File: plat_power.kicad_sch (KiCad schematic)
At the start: 56 parts, among them Con2 DG125-5.0-02P-14-00A(H), U1 LD39050PU33R, U2 TPS5450, U3 TPS5450, U4 TPS5450, con3 KF202

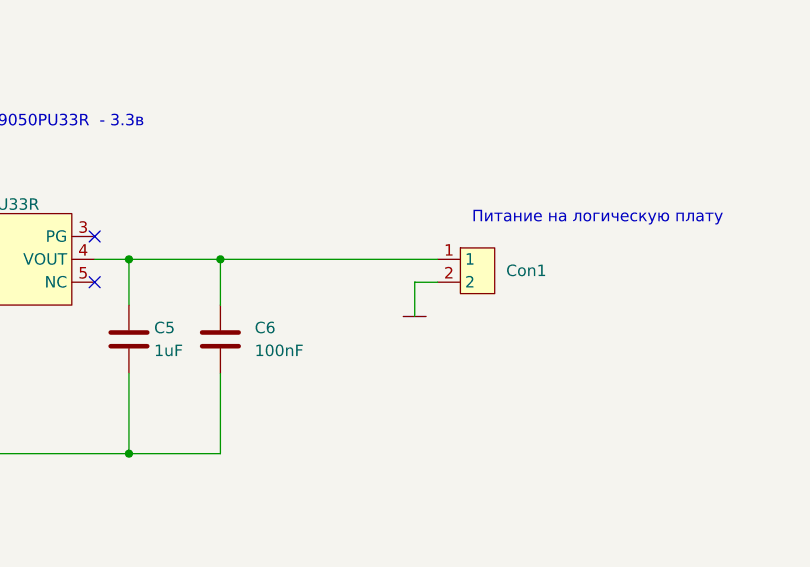
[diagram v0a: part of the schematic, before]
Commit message: Add files via upload
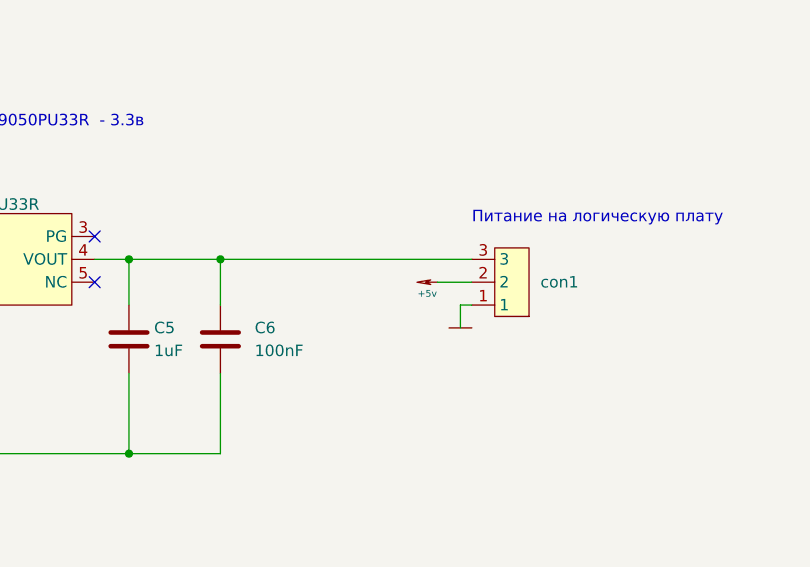
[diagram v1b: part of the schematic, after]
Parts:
- removed Con1: (no value), Connector_PinHeader_1.00mm:PinHeader_1x02_P1.00mm_Vertical, symbol MyLIB:Con_power
- added con1: (no value), Connector_PinHeader_1.00mm:PinHeader_1x03_P1.00mm_Vertical, symbol MyLIB:con_3
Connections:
- net +5v: now also con1.2
- net GND: now also con1.1
- net at C5.1, C6.1, U1.4 (VOUT): now also con1.3
